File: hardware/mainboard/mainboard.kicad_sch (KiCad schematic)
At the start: 1 part, among them J1 EXT

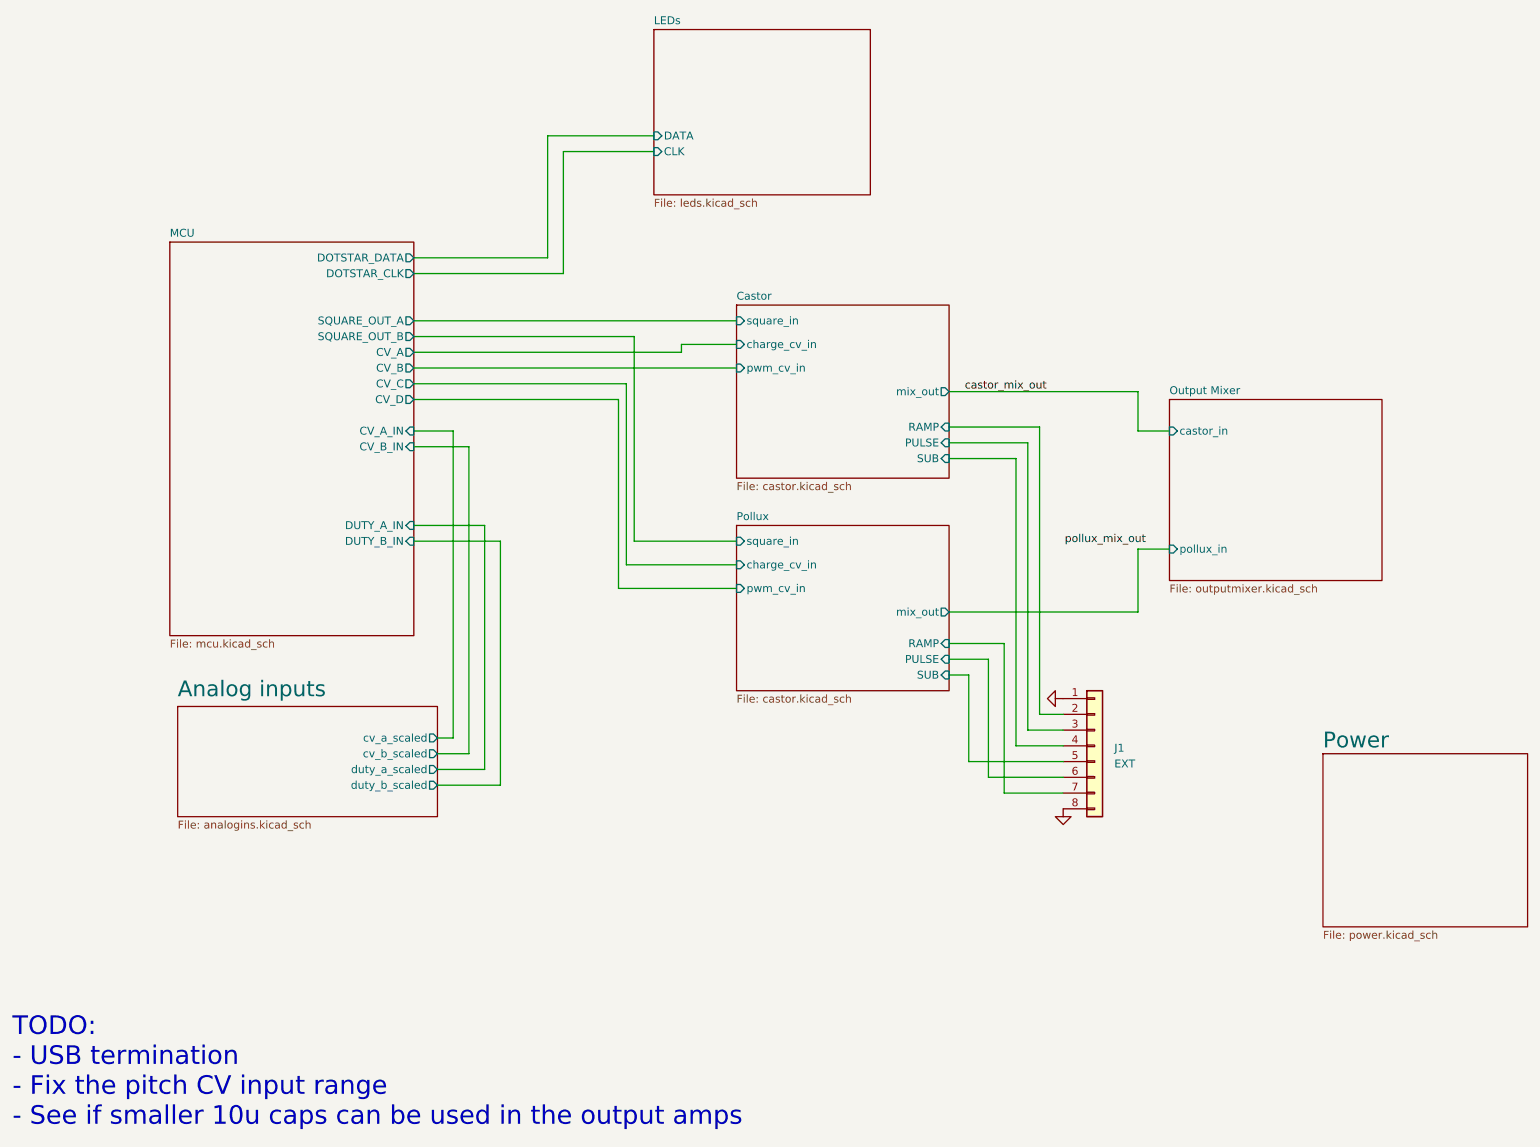
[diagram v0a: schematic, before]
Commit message: More schematic cleanup - nearly done!
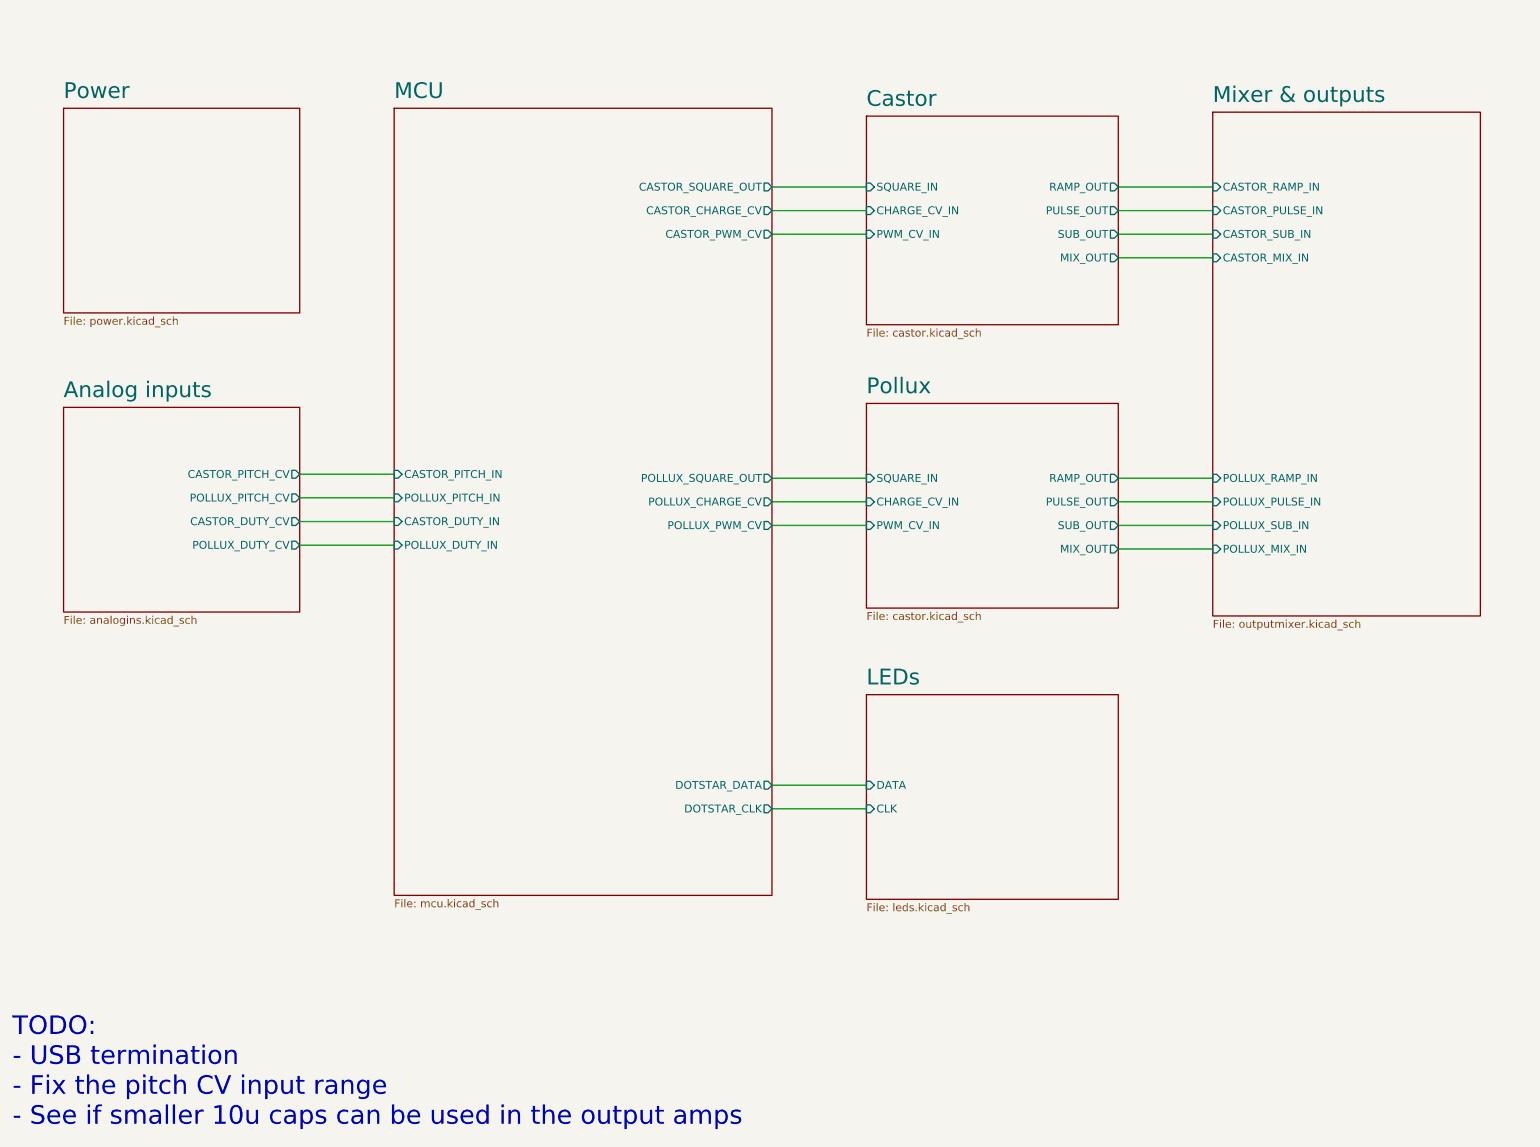
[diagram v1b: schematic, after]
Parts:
- removed J1: EXT, Connector_JST:JST_GH_BM08B-GHS-TBT_1x08-1MP_P1.25mm_Vertical, symbol Connector_Generic:Conn_01x08
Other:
- sheet Output Mixer renamed Mixer & outputs
- sheet Analog inputs ports: added CASTOR_DUTY_CV, CASTOR_PITCH_CV, POLLUX_DUTY_CV, POLLUX_PITCH_CV; removed cv_a_scaled, cv_b_scaled, duty_a_scaled, duty_b_scaled
- sheet Castor ports: added CHARGE_CV_IN, MIX_OUT, PULSE_OUT, PWM_CV_IN, RAMP_OUT, SQUARE_IN, SUB_OUT; removed PULSE, RAMP, SUB, charge_cv_in, mix_out, pwm_cv_in, square_in
- sheet MCU ports: added CASTOR_CHARGE_CV, CASTOR_DUTY_IN, CASTOR_PITCH_IN, CASTOR_PWM_CV, CASTOR_SQUARE_OUT, POLLUX_CHARGE_CV, POLLUX_DUTY_IN, POLLUX_PITCH_IN, POLLUX_PWM_CV, POLLUX_SQUARE_OUT; removed CV_A, CV_A_IN, CV_B, CV_B_IN, CV_C, CV_D, DUTY_A_IN, DUTY_B_IN, SQUARE_OUT_A, SQUARE_OUT_B
- sheet Mixer & outputs ports: added CASTOR_MIX_IN, CASTOR_PULSE_IN, CASTOR_RAMP_IN, CASTOR_SUB_IN, POLLUX_MIX_IN, POLLUX_PULSE_IN, POLLUX_RAMP_IN, POLLUX_SUB_IN; removed castor_in, pollux_in
- sheet Pollux ports: added CHARGE_CV_IN, MIX_OUT, PULSE_OUT, PWM_CV_IN, RAMP_OUT, SQUARE_IN, SUB_OUT; removed PULSE, RAMP, SUB, charge_cv_in, mix_out, pwm_cv_in, square_in
